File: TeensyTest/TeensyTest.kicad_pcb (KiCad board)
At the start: 2 copper layers, 45 x 34 mm, 32 parts, among them J2 Conn_01x08_Female, J3 Conn_01x04_Female, P1 USB_C_Plug_USB2.0, SW1 SW_Push, SW2 SW_Push, U1 AP2114H, U2 MK20DX256VLH7, U3 MKL02Z32VFG4, Y1 Crystal_GND24

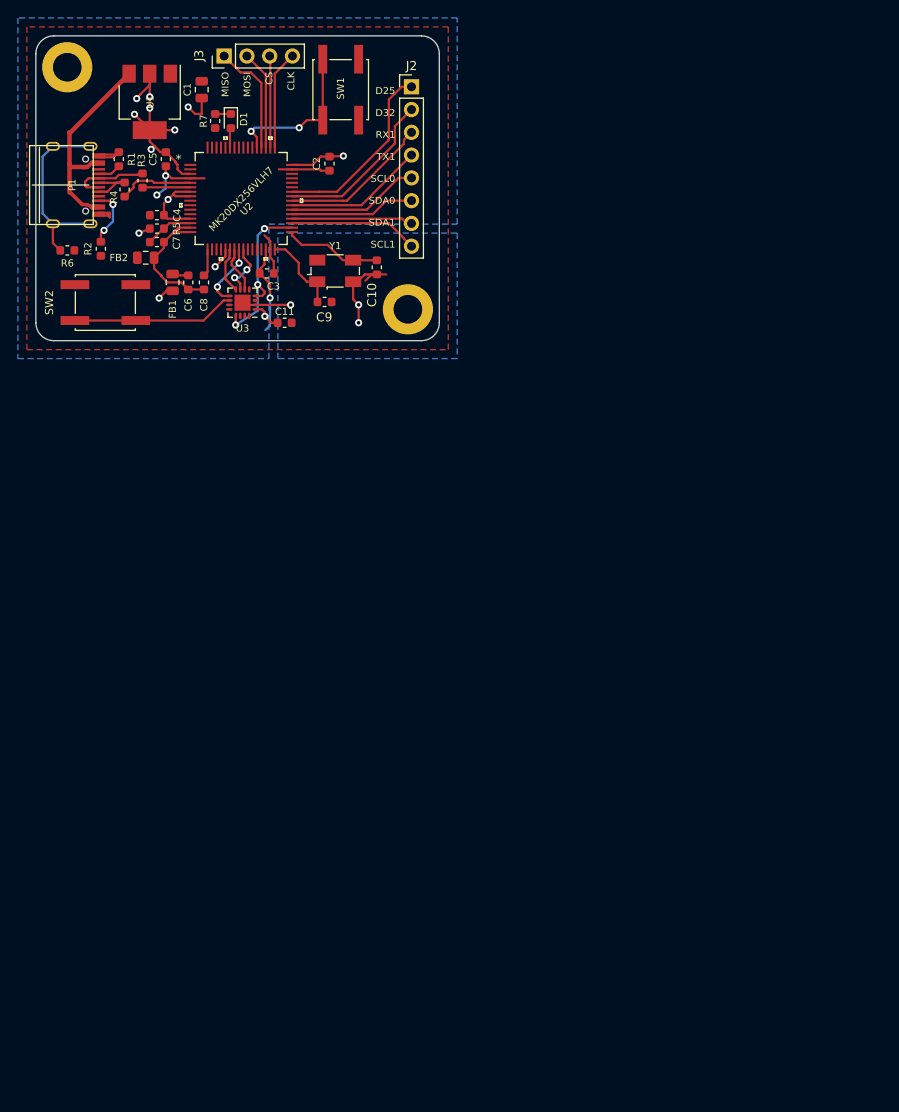
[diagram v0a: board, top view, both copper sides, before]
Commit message: Initial commit
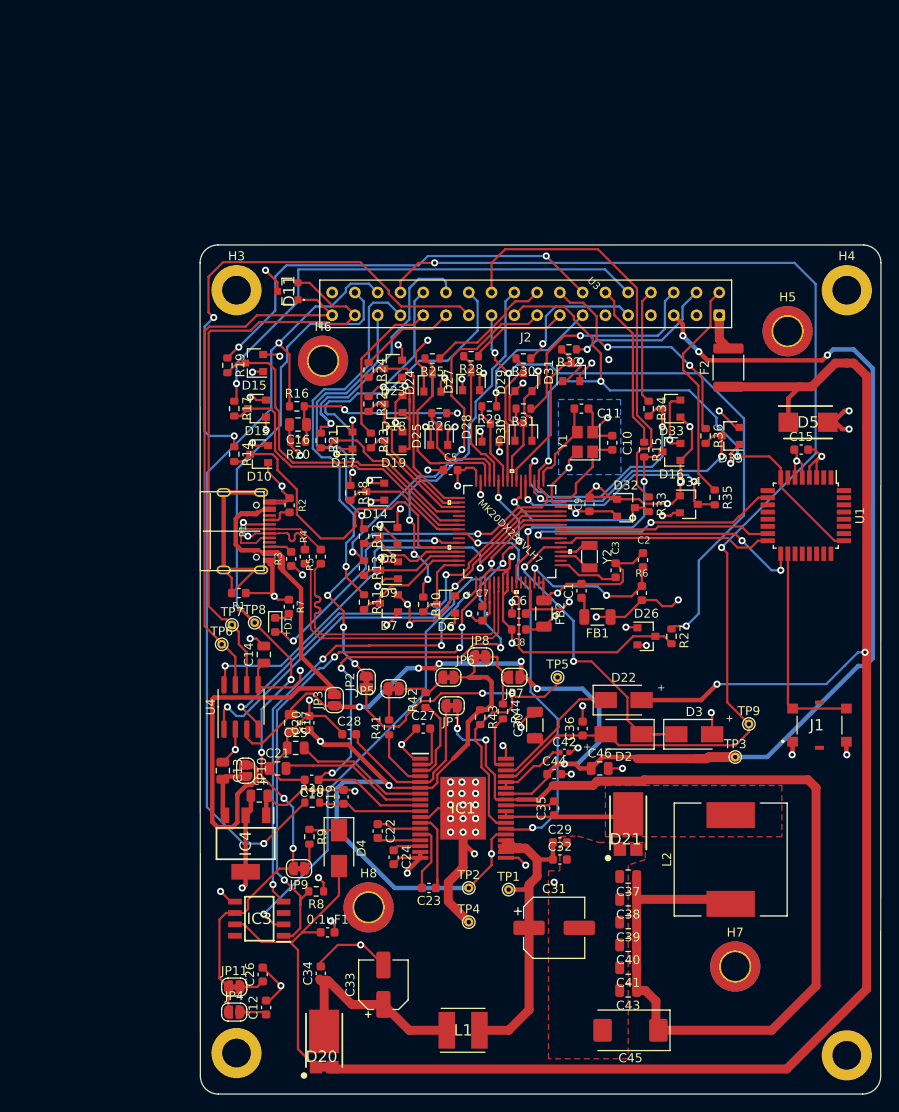
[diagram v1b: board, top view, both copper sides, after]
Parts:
- removed the C3 at (41.4, 62.4)
- removed J3: Conn_01x04_Female, Connector_PinHeader_2.54mm:PinHeader_1x04_P2.54mm_Vertical
- removed SW1, SW2: SW_Push, Button_Switch_SMD:SW_SPST_EVQQ2
- removed the U1 at (28.3, 43.2)
- added 0.1uF1: C, Capacitor_SMD:C_0603_1608Metric, F.Cu at (48.1, 135.9)
- added C12: 220pF, Capacitor_SMD:C_0603_1608Metric, F.Cu at (41.3, 144.2)
- added C13: 10uF, Capacitor_SMD:C_0805_2012Metric, F.Cu at (36.5, 117.8)
- added C14: 0.1uF, Capacitor_SMD:C_0805_2012Metric, F.Cu at (41.0, 104.9)
- added C15: 0.1uF, Capacitor_SMD:C_0603_1608Metric, F.Cu at (101.0, 82.0)
- added C16: 0.1uF, Capacitor_SMD:C_0805_2012Metric, F.Cu at (44.8, 79.2)
- added C17: 0.1uF, Capacitor_SMD:C_0805_2012Metric, F.Cu at (44.1, 112.5)
- added C18: 10nF/50V, Capacitor_SMD:C_0603_1608Metric, F.Cu at (46.4, 118.8)
- added C19: 0.1uF/50V, Capacitor_SMD:C_0603_1608Metric, F.Cu at (49.9, 120.7)
- added C20: 1uF/10V, Capacitor_SMD:C_0603_1608Metric, F.Cu at (46.1, 112.5)
- added C21: 4.7uF/25V, Capacitor_SMD:C_0805_2012Metric, F.Cu at (42.6, 117.6)
- added C22: 0.1uF/16V, Capacitor_SMD:C_0603_1608Metric, F.Cu at (53.7, 124.6)
- added C23: 0.1uF/16V, Capacitor_SMD:C_0603_1608Metric, F.Cu at (59.4, 130.9)
- added C24: 0.22uF/25V, Capacitor_SMD:C_0603_1608Metric, F.Cu at (55.5, 127.5)
- added C25: 4.7uF/25V, Capacitor_SMD:C_0805_2012Metric, F.Cu at (44.6, 115.3)
- added C26: 1nF, Capacitor_SMD:C_0603_1608Metric, F.Cu at (40.9, 140.6)
- added C27: 1n/10V, Capacitor_SMD:C_0603_1608Metric, F.Cu at (58.8, 113.1)
- added C28: 0.1uF/16V, Capacitor_SMD:C_0603_1608Metric, F.Cu at (50.6, 113.8)
- added C29: 0.1uF/50V, Capacitor_SMD:C_0603_1608Metric, F.Cu at (74.0, 125.8)
- added C30: 470nF/50V, Capacitor_SMD:C_1206_3216Metric, F.Cu at (71.3, 112.7)
- added C31: 10uF/50V, Capacitor_SMD:CP_Elec_6.3x5.4, F.Cu at (73.4, 135.3)
- added C32: 0.1uF/50V, Capacitor_SMD:C_0603_1608Metric, F.Cu at (74.0, 127.7)
- added C33: 10uF/50V, Capacitor_SMD:CP_Elec_5x5.3, F.Cu at (54.4, 141.7)
- added C34: 0.1uF/50V, Capacitor_SMD:C_0603_1608Metric, F.Cu at (47.4, 140.4)
- added C35: 0.1uF/10V, Capacitor_SMD:C_0603_1608Metric, F.Cu at (73.4, 122.0)
- added C36: 1uF/10V, Capacitor_SMD:C_0603_1608Metric, F.Cu at (76.6, 113.1)
- added C37: 4.7uF/16V, Capacitor_SMD:C_0805_2012Metric, F.Cu at (81.7, 129.6)
- added C38: 4.7uF/16V, Capacitor_SMD:C_0805_2012Metric, F.Cu at (81.7, 132.2)
- added C39: 4.7uF/16V, Capacitor_SMD:C_0805_2012Metric, F.Cu at (81.7, 134.7)
- added C40: 4.7uF/16V, Capacitor_SMD:C_0805_2012Metric, F.Cu at (81.7, 137.3)
- added C41: 4.7uF/16V, Capacitor_SMD:C_0805_2012Metric, F.Cu at (81.7, 139.8)
- added C42: 220nF, Capacitor_SMD:C_0402_1005Metric, F.Cu at (74.6, 115.8)
- added C43: 4.7uF/16V, Capacitor_SMD:C_0805_2012Metric, F.Cu at (81.7, 142.3)
- added C44: 10uF/10V, Capacitor_SMD:C_0603_1608Metric, F.Cu at (73.4, 118.2)
- added C45: 47uF/16V, Capacitor_Tantalum_SMD:CP_EIA-7343-31_Kemet-D, F.Cu at (81.9, 146.8)
- added C46: 1uF/10V, Capacitor_SMD:C_0805_2012Metric, F.Cu at (78.5, 117.6)
- added C6: 0.1uF, Capacitor_SMD:C_0603_1608Metric, F.Cu at (69.5, 100.3)
- added D10: BAS40-04, Package_TO_SOT_SMD:SOT-23, F.Cu at (40.5, 82.5)
- added D11: SM24CANB-02HTG, SamacSys_Parts:SM24CANB02HTG, F.Cu at (43.7, 64.4)
- added D13: BAS40-04, Package_TO_SOT_SMD:SOT-23, F.Cu at (40.3, 77.4)
- added D14: BAS40-04, Package_TO_SOT_SMD:SOT-23, F.Cu at (53.5, 86.7)
- added D15: BAS40-04, Package_TO_SOT_SMD:SOT-23, F.Cu at (40.0, 72.4)
- added D16: BAS40-04, Package_TO_SOT_SMD:SOT-23, F.Cu at (86.5, 82.3)
- added D17: BAS40-04, Package_TO_SOT_SMD:SOT-23, F.Cu at (49.9, 81.0)
- added D18: BAS40-04, Package_TO_SOT_SMD:SOT-23, F.Cu at (55.5, 76.9)
- added D19: BAS40-04, Package_TO_SOT_SMD:SOT-23, F.Cu at (55.5, 81.0)
- added D2: D, Diode_SMD:D_SMA, F.Cu at (81.2, 113.8)
- added D20: SBR12U100P5-13, SamacSys_Parts:POWERDI5, F.Cu at (47.8, 146.9)
- added D21: SBR12U100P5-13, SamacSys_Parts:POWERDI5, F.Cu at (81.7, 122.6)
- added D22: D, Diode_SMD:D_SMA, F.Cu at (81.2, 109.9)
- added D23: BAS40-04, Package_TO_SOT_SMD:SOT-23, F.Cu at (55.4, 73.0)
- added D24: BAS40-04, Package_TO_SOT_SMD:SOT-23, F.Cu at (59.8, 74.5)
- added D25: BAS40-04, Package_TO_SOT_SMD:SOT-23, F.Cu at (60.6, 80.5)
- added D26: BAS40-04, Package_TO_SOT_SMD:SOT-23, F.Cu at (83.7, 102.8)
- added D27: BAS40-04, Package_TO_SOT_SMD:SOT-23, F.Cu at (64.1, 74.4)
- added D28: BAS40-04, Package_TO_SOT_SMD:SOT-23, F.Cu at (66.3, 80.1)
- added D29: BAS40-04, Package_TO_SOT_SMD:SOT-23, F.Cu at (70.0, 74.5)
- added D3: D, Diode_SMD:D_SMA, F.Cu at (89.0, 113.8)
- added D30: BAS40-04, Package_TO_SOT_SMD:SOT-23, F.Cu at (70.0, 80.0)
- added D31: BAS40-04, Package_TO_SOT_SMD:SOT-23, F.Cu at (75.3, 73.4)
- added D32: BAS40-04, Package_TO_SOT_SMD:SOT-23, F.Cu at (81.4, 88.5)
- added D33: BAS40-04, Package_TO_SOT_SMD:SOT-23, F.Cu at (86.5, 77.4)
- added D34: BAS40-04, Package_TO_SOT_SMD:SOT-23, F.Cu at (88.4, 88.1)
- added D35: BAS40-04, Package_TO_SOT_SMD:SOT-23, F.Cu at (93.1, 80.5)
- added D4: D, Diode_SMD:D_SMA, F.Cu at (49.4, 126.5)
- added D5: SMBJ33A, SamacSys_Parts:DIOM5436X244N, F.Cu at (101.7, 79.0)
- added D6: BAS40-04, Package_TO_SOT_SMD:SOT-23, F.Cu at (61.3, 99.3)
- added D7: BAS40-04, Package_TO_SOT_SMD:SOT-23, F.Cu at (55.0, 99.2)
- added D8: BAS40-04, Package_TO_SOT_SMD:SOT-23, F.Cu at (54.9, 91.7)
- added D9: BAS40-04, Package_TO_SOT_SMD:SOT-23, F.Cu at (55.0, 95.5)
- added F2: Fuse, Fuse:Fuse_1812_4532Metric, F.Cu at (92.8, 72.9)
- added H3: MountingHole, MountingHole:MountingHole_3.2mm_M3_DIN965_Pad, F.Cu at (38.0, 64.2)
- added H4: MountingHole, MountingHole:MountingHole_3.2mm_M3_DIN965_Pad, F.Cu at (106.1, 64.2)
- added H5: MountingHole_Pad, MountingHole:MountingHole_3.2mm_M3_DIN965_Pad_TopBottom, F.Cu at (99.4, 68.8)
- added H6: MountingHole_Pad, MountingHole:MountingHole_3.2mm_M3_DIN965_Pad_TopBottom, F.Cu at (47.6, 72.1)
- added H7: MountingHole_Pad, MountingHole:MountingHole_3.2mm_M3_DIN965_Pad_TopBottom, F.Cu at (93.6, 139.7)
- added H8: MountingHole_Pad, MountingHole:MountingHole_3.2mm_M3_DIN965_Pad_TopBottom, F.Cu at (52.7, 133.1)
- added IC1: TLE73683EXUMA2, SamacSys_Parts:SOP65P1030X255-37N, F.Cu at (63.3, 122.0)
- added IC3: TLIN2029DRQ1, SamacSys_Parts:SOIC127P600X175-8N, F.Cu at (40.5, 134.3)
- added IC4: LM1117MPX-3.3_NOPB, SamacSys_Parts:SOT230P700X180-4N, F.Cu at (39.0, 126.0)
- added J1: 431151015826, SamacSys_Parts:431151015826, F.Cu at (103.0, 112.7)
- added JP1: SolderJumper_2_Bridged!!!, Jumper:SolderJumper-2_P1.3mm_Bridged_RoundedPad1.0x1.5mm, F.Cu at (62.0, 110.6)
- added JP10: SolderJumper_2_Bridged, Jumper:SolderJumper-2_P1.3mm_Open_RoundedPad1.0x1.5mm, F.Cu at (39.0, 117.8)
- added JP11: Jumper_2_Closed, Jumper:SolderJumper-2_P1.3mm_Bridged_RoundedPad1.0x1.5mm, F.Cu at (37.7, 142.0)
- added JP2: SolderJumper_2_Bridged, Jumper:SolderJumper-2_P1.3mm_Bridged_RoundedPad1.0x1.5mm, F.Cu at (52.5, 107.9)
- added JP3: SolderJumper_2_Bridged, Jumper:SolderJumper-2_P1.3mm_Open_RoundedPad1.0x1.5mm, F.Cu at (48.9, 109.9)
- added JP4: Jumper_2_Open, Jumper:SolderJumper-2_P1.3mm_Open_RoundedPad1.0x1.5mm, F.Cu at (37.7, 144.7)
- added JP5: SolderJumper_2_Bridged, Jumper:SolderJumper-2_P1.3mm_Bridged_RoundedPad1.0x1.5mm, F.Cu at (55.5, 108.7)
- added JP6: SolderJumper_2_Bridged, Jumper:SolderJumper-2_P1.3mm_Bridged_RoundedPad1.0x1.5mm, F.Cu at (61.6, 107.4)
- added JP7: SolderJumper_2_Open, Jumper:SolderJumper-2_P1.3mm_Open_RoundedPad1.0x1.5mm, F.Cu at (69.0, 107.4)
- added JP8: SolderJumper_2_Bridged, Jumper:SolderJumper-2_P1.3mm_Bridged_RoundedPad1.0x1.5mm, F.Cu at (65.2, 105.1)
- added JP9: Jumper_2_Closed, Jumper:SolderJumper-2_P1.3mm_Bridged_RoundedPad1.0x1.5mm, F.Cu at (45.0, 128.7)
- added L1: 10 μH/2.1 A, SamacSys_Parts:LQH5BPN100M38L, F.Cu at (63.3, 146.8)
- added L2: 33 μH/2.1 A, Inductor_SMD:L_12x12mm_H6mm, F.Cu at (93.1, 127.7)
- added R10: 4.7K, Resistor_SMD:R_0603_1608Metric, F.Cu at (58.8, 99.3)
- added R11: 4.7K, Resistor_SMD:R_0603_1608Metric, F.Cu at (52.2, 99.0)
- added R12: 4.7K, Resistor_SMD:R_0603_1608Metric, F.Cu at (52.2, 91.7)
- added R13: 4.7K, Resistor_SMD:R_0603_1608Metric, F.Cu at (52.2, 95.2)
- added R14: 4.7K, Resistor_SMD:R_0603_1608Metric, F.Cu at (37.7, 82.5)
- added R15: 4.7K, Resistor_SMD:R_0603_1608Metric, F.Cu at (83.4, 82.0)
- added R16: 180K, Resistor_SMD:R_0603_1608Metric, F.Cu at (44.7, 77.2)
- added R17: 4.7K, Resistor_SMD:R_0603_1608Metric, F.Cu at (37.7, 77.4)
- added R18: 4.7K, Resistor_SMD:R_0603_1608Metric, F.Cu at (50.7, 86.8)
- added R19: 4.7K, Resistor_SMD:R_0603_1608Metric, F.Cu at (37.0, 72.6)
- added R20: 68K, Resistor_SMD:R_0603_1608Metric, F.Cu at (44.8, 81.1)
- added R21: 4.7K, Resistor_SMD:R_0603_1608Metric, F.Cu at (47.4, 81.0)
- added R22: 4.7K, Resistor_SMD:R_0603_1608Metric, F.Cu at (52.7, 76.9)
- added R23: 4.7K, Resistor_SMD:R_0603_1608Metric, F.Cu at (53.0, 81.0)
- added R24: 4.7K, Resistor_SMD:R_0603_1608Metric, F.Cu at (52.7, 73.1)
- added R25: 4.7K, Resistor_SMD:R_0603_1608Metric, F.Cu at (59.8, 71.8)
- added R26: 4.7K, Resistor_SMD:R_0603_1608Metric, F.Cu at (60.6, 77.9)
- added R27: 4.7K, Resistor_SMD:R_0603_1608Metric, F.Cu at (86.5, 102.8)
- added R28: 4.7K, Resistor_SMD:R_0603_1608Metric, F.Cu at (64.1, 71.6)
- added R29: 4.7K, Resistor_SMD:R_0603_1608Metric, F.Cu at (66.2, 77.2)
- added R30: 4.7K, Resistor_SMD:R_0603_1608Metric, F.Cu at (70.0, 71.8)
- added R31: 4.7K, Resistor_SMD:R_0603_1608Metric, F.Cu at (70.0, 77.4)
- added R32: 4.7K, Resistor_SMD:R_0603_1608Metric, F.Cu at (75.1, 70.8)
- added R33: 4.7K, Resistor_SMD:R_0603_1608Metric, F.Cu at (84.0, 88.1)
- added R34: 4.7K, Resistor_SMD:R_0603_1608Metric, F.Cu at (84.0, 77.4)
- added R35: 4.7K, Resistor_SMD:R_0603_1608Metric, F.Cu at (91.3, 87.3)
- added R36: 4.7K, Resistor_SMD:R_0603_1608Metric, F.Cu at (90.3, 80.5)
- added R40: 10K, Resistor_SMD:R_0603_1608Metric, F.Cu at (46.4, 121.4)
- added R41: 10K, Resistor_SMD:R_0603_1608Metric, F.Cu at (55.0, 113.0)
- added R42: 10K, Resistor_SMD:R_0603_1608Metric, F.Cu at (59.1, 109.9)
- added R43: 10K, Resistor_SMD:R_0603_1608Metric, F.Cu at (65.2, 111.9)
- added R44: 10K, Resistor_SMD:R_0603_1608Metric, F.Cu at (67.7, 111.2)
- added R8: 4K7, Resistor_SMD:R_0603_1608Metric, F.Cu at (46.9, 131.3)
- added R9: 1K, Resistor_SMD:R_0603_1608Metric, F.Cu at (46.1, 125.2)
- added TP1: TestPoint, TestPoint:TestPoint_THTPad_D1.0mm_Drill0.5mm, F.Cu at (68.3, 131.1)
- added TP2: TestPoint, TestPoint:TestPoint_THTPad_D1.0mm_Drill0.5mm, F.Cu at (63.9, 130.9)
- added TP3: TestPoint, TestPoint:TestPoint_THTPad_D1.0mm_Drill0.5mm, F.Cu at (93.6, 116.3)
- added TP4: TestPoint, TestPoint:TestPoint_THTPad_D1.0mm_Drill0.5mm, F.Cu at (63.9, 134.7)
- added TP5: TestPoint, TestPoint:TestPoint_THTPad_D1.0mm_Drill0.5mm, F.Cu at (73.8, 107.4)
- added TP6: TestPoint, TestPoint:TestPoint_THTPad_D1.0mm_Drill0.5mm, F.Cu at (36.3, 103.7)
- added TP7: TestPoint, TestPoint:TestPoint_THTPad_D1.0mm_Drill0.5mm, F.Cu at (37.5, 101.6)
- added TP8: TestPoint, TestPoint:TestPoint_THTPad_D1.0mm_Drill0.5mm, F.Cu at (40.0, 101.3)
- added TP9: TestPoint, TestPoint:TestPoint_THTPad_D1.0mm_Drill0.5mm, F.Cu at (95.1, 112.6)
- added U4: MCP2562-E-SN, Package_SO:SOIC-8_3.9x4.9mm_P1.27mm, F.Cu at (38.5, 110.7)
- added Y2: Crystal, Crystal:Crystal_SMD_3215-2Pin_3.2x1.5mm, F.Cu at (77.3, 93.9)
- C1: renamed from C6; footprint Resistor_SMD:R_0603_1608Metric -> Capacitor_SMD:C_0603_1608Metric
- FB1, FB2: footprint Resistor_SMD:R_0805_2012Metric -> Resistor_SMD:R_1206_3216Metric
- J2: value Conn_01x08_Female -> Conn_02x18_Odd_Even; footprint Connector_PinHeader_2.54mm:PinHeader_1x08_P2.54mm_Vertical -> Connector_Samtec_HLE_THT:Samtec_HLE-118-02-xx-DV-TE_2x18_P2.54mm_Horizontal
- U1: renamed from U3; footprint Package_DFN_QFN:QFN-16-1EP_3x3mm_P0.5mm_EP1.8x1.8mm -> Package_QFP:TQFP-32_7x7mm_P0.8mm
- Y1: footprint Crystal:Crystal_SMD_Abracon_ABM3B-4Pin_5.0x3.2mm -> Crystal:Crystal_SMD_3225-4Pin_3.2x2.5mm
- moved H1 111.6 mm to (38.0, 149.3)
- moved H2 96.5 mm to (106.1, 149.6)
- moved C4 79.0 mm to (40.5, 120.6), turned to 180 degrees
- moved R6 67.7 mm to (83.2, 98.0), turned to 270 degrees
- moved U1 67.2 mm to (101.5, 89.4), turned to 270 degrees
- moved C8 65.6 mm to (69.5, 102.1), turned to 180 degrees
- moved C2 64.8 mm to (83.3, 94.3), turned to 90 degrees
- moved FB1 60.3 mm to (78.2, 100.7), turned to 180 degrees
- moved FB2 59.6 mm to (72.3, 100.3), turned to 270 degrees
- moved C7 57.4 mm to (65.4, 100.3), turned to 90 degrees
- moved D1 56.4 mm to (42.3, 101.6)
- moved C3 56.0 mm to (80.3, 95.5), turned to 270 degrees
- moved C1 55.7 mm to (76.5, 97.8), turned to 90 degrees
- moved R7 54.8 mm to (43.8, 99.5), turned to 90 degrees
- moved U3 47.7 mm to (68.5, 91.2), turned to 90 degrees
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- renumbered C9 to C10, C10 to C11, C7 to C2, C8 to C3, C1 to C4, C2 to C5, C4 to C7, C5 to C8, C11 to C9, R6 to R1, R1 to R2, R2 to R3, R3 to R4, R4 to R5, R5 to R6, U2 to U3
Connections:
- net /DM renamed /D_N
- net /DP renamed /D_P
- C10 pad 2: GND -> GND1
- C11 pad 2: GND -> GND1
- J2 pad 1: /D25 -> +12V
- J2 pad 2: /D32 -> /D19
- J2 pad 3: /D1 -> +3V3
- J2 pad 5: /D18 -> +5V
- J2 pad 6: /D19 -> /D1
- J2 pad 7: /D17 -> GND
- J2 pad 8: /D16 -> /D17
- P1 pad A8: (no net) -> Net-(P1-PadA8)
- P1 pad B8: (no net) -> Net-(P1-PadB8)
- U1 pad 1: +3V3 -> Net-(U1-Pad1)
- U1 pad 10: Net-(SW2-Pad1) -> Net-(U1-Pad10)
- U1 pad 11: (no net) -> Net-(U1-Pad11)
- U1 pad 12: (no net) -> Net-(U1-Pad12)
- U1 pad 13: RESET_B -> Net-(U1-Pad13)
- U1 pad 14: (no net) -> Net-(U1-Pad14)
- U1 pad 15: (no net) -> Net-(U1-Pad15)
- U1 pad 16: (no net) -> Net-(U1-Pad16)
- U1 pad 17: GND -> Net-(U1-Pad17)
- U1 pad 2: GND -> Net-(U1-Pad2)
- U1 pad 3: (no net) -> +3V3
- U1 pad 4: RESET_B -> +3V3
- U1 pad 5: (no net) -> GND
- U1 pad 6: Net-(U2-Pad23) -> GND
- U1 pad 7: Net-(U2-Pad25) -> Net-(U1-Pad7)
- U1 pad 8: Net-(U2-Pad22) -> RESET_B
- U1 pad 9: Net-(U2-Pad24) -> Net-(U1-Pad9)
- U3 pad 1: (no net) -> /31
- U3 pad 10: (no net) -> /A11_1
- U3 pad 11: (no net) -> /A12
- U3 pad 12: (no net) -> /A13
- U3 pad 18: (no net) -> /DAC_A14
- U3 pad 19: (no net) -> Net-(U3-Pad19)
- U3 pad 2: (no net) -> /26
- U3 pad 20: (no net) -> Net-(U3-Pad20)
- U3 pad 21: +3V3 -> Net-(D2-Pad1)
- U3 pad 22: Net-(U2-Pad22) -> Net-(U1-Pad16)
- U3 pad 23: Net-(U2-Pad23) -> Net-(U1-Pad10)
- U3 pad 24: Net-(U2-Pad24) -> Net-(U1-Pad17)
- U3 pad 25: Net-(U2-Pad25) -> Net-(U1-Pad15)
- U3 pad 26: (no net) -> /33
- U3 pad 27: (no net) -> /24
- U3 pad 28: (no net) -> /CTX
- U3 pad 29: (no net) -> /CRX
- U3 pad 31: GND -> GND1
- U3 pad 35: /D16 -> /sheet60791461/1
- U3 pad 36: /D17 -> /sheet6079145F/1
- U3 pad 37: /D19 -> /sheet60791460/1
- U3 pad 38: /D18 -> /sheet6079145E/1
- U3 pad 39: /D0 -> /sheet6079145D/1
- U3 pad 40: /D1 -> /sheet6079145C/1
- U3 pad 41: /D32 -> /sheet6079145B/1
- U3 pad 42: /D25 -> /sheet60705A03/1
- U3 pad 43: (no net) -> /15_A1
- U3 pad 44: (no net) -> /sheet60705A02/1
- U3 pad 45: (no net) -> /sheet60705A00/1
- U3 pad 46: (no net) -> /sheet607059FF/1
- U3 pad 49: /D10 -> /sheet606FF68E/1
- U3 pad 50: /D13 -> /sheet606FF68C/1
- U3 pad 51: /D11 -> /sheet606FF68D/1
- U3 pad 52: /D12 -> /sheet606FF68B/1
- U3 pad 54: (no net) -> /sheet606F9355/1
- U3 pad 55: (no net) -> /sheet606F9353/1
- U3 pad 56: (no net) -> /sheet606F9354/1
- U3 pad 57: (no net) -> /2
- U3 pad 58: (no net) -> /14_A0
- U3 pad 60: (no net) -> /sheet606D7D50/1
- U3 pad 61: (no net) -> /sheet6068C209/1
- U3 pad 62: (no net) -> /sheet606C2E9F/1
- U3 pad 63: (no net) -> /sheet60685D3E/1
- U3 pad 64: (no net) -> /InputProtection/1
- U3 pad 9: (no net) -> /A10_1
- Y1 pad 2: GND -> GND1
- Y1 pad 4: GND -> GND1
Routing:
- net VCC: track 0.00 -> 217.6 mm, vias 0 -> 2
- net GND: track 43.6 -> 252.0 mm, vias 5 -> 70
- net +5V: track 0.00 -> 183.2 mm, vias 0 -> 9
- net +3V3: track 60.9 -> 236.0 mm, vias 14 -> 37
- net /TLE73683EXUMA2/BUCK: track 0.00 -> 145.7 mm, vias 0 -> 2
- net /Q_STBY: track 0.00 -> 135.1 mm, vias 0 -> 2
- net /LIN: track 0.00 -> 105.9 mm, vias 0 -> 4
- net RESET_B: track 18.9 -> 114.0 mm, vias 3 -> 7
- net /IGN: track 0.00 -> 91.5 mm, vias 0 -> 2
- net /15_A1: track 0.00 -> 69.7 mm, vias 0 -> 6
- net /CANL: track 0.00 -> 67.4 mm
- net /A10: track 0.00 -> 64.4 mm, vias 0 -> 3
- net /33: track 0.00 -> 63.0 mm, vias 0 -> 2
- net /26: track 0.00 -> 60.9 mm, vias 0 -> 4
- net /CANH: track 0.00 -> 60.3 mm
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- added copper zone on In2.Cu, net +3V3
- added copper zone on F.Cu, net /TLE73683EXUMA2/SW_1
- added copper zone on In1.Cu, net GND
- added copper zone on B.Cu, net GND1
- removed copper zone on B.Cu, net +3V3
- removed copper zone on B.Cu, net GND
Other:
- board size 45 x 34 mm -> 75.9 x 94.7 mm
- copper layers 2 -> 4
- rule pad_to_mask_clearance: 0.051 -> 0
- board text added: "+"
- board text removed: "D25 D32 RX1 TX1 SCL0 SDA0 SDA1 SCL1"
- board text removed: "MISO MOSI CS CLK"
